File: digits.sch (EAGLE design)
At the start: 49 parts, among them IC1 STP16CP05 / STP16CPC26, IC2 STP16CP05 / STP16CPC26, IC3 ATMEGA32U4QFN, IC4 ATMEGA32U4TQFP-44, J1 POWER_JACKPTH_LOCK, J2 ACCESSORY, X1 CRYSTALHC49

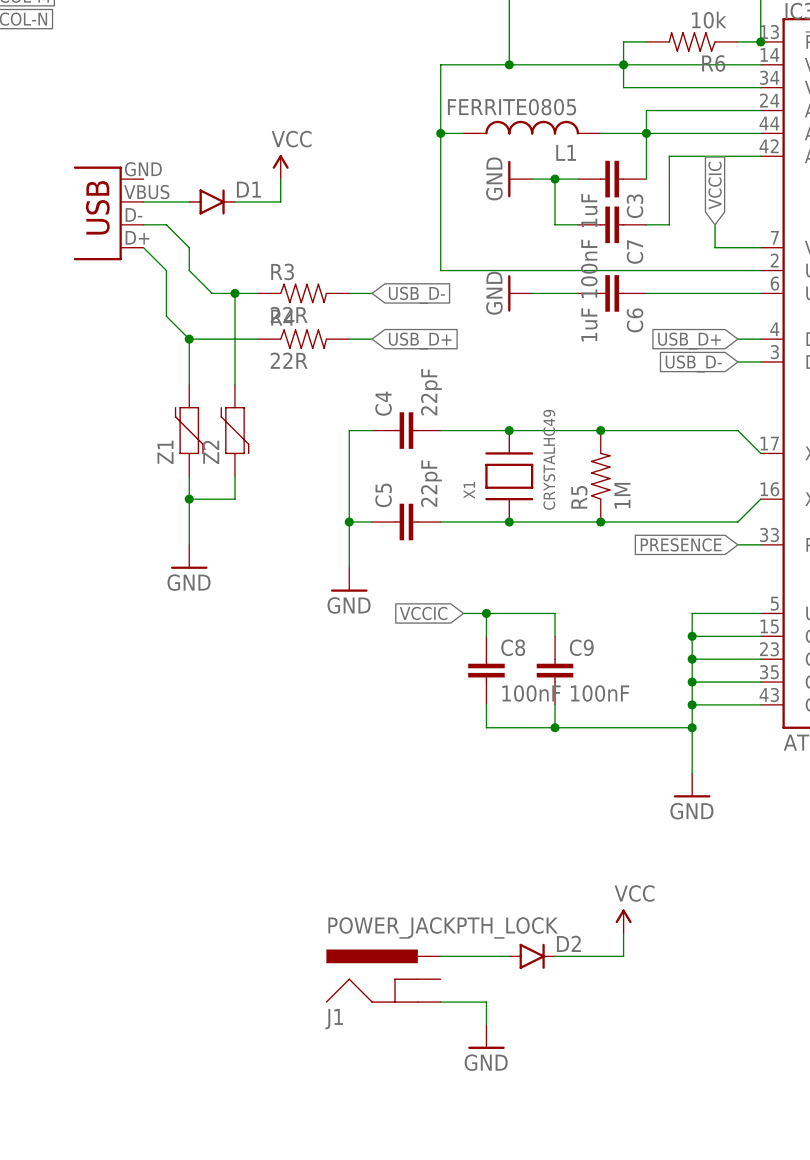
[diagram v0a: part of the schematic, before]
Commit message: finished BOM
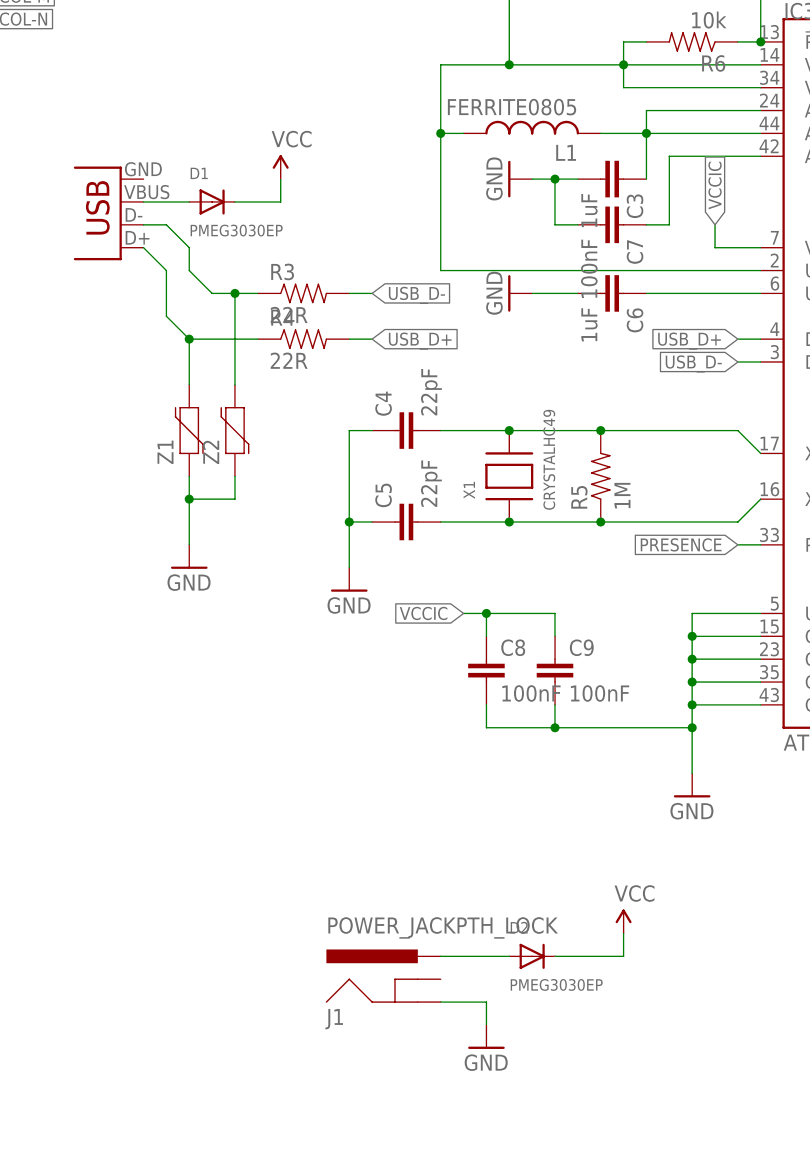
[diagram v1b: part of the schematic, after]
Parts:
- C1, C2, C7, C8, C9: PARTNO (none) -> C0805C104K5RACTU
- C3, C6: PARTNO (none) -> CL21B105KBFNNNE
- C4, C5: PARTNO (none) -> C0805C220J5GACTU
- D1, D2: value (none) -> PMEG3030EP; device SparkFun-DiscreteSemi:DIODESOD -> digits:DIODESOD-128; PARTNO (none) -> PMEG3030EP-115
- IC1, IC2: PARTNO (none) -> STP16CPC26MTR
- IC3: PARTNO (none) -> ATMEGA32U4-MUR
- IC4: PARTNO (none) -> ATMEGA32U4-AU
- J1: PARTNO (none) -> PJ-202A
- J2: PARTNO (none) -> SFH11-PBPC-D13-ST-BK
- JP1: PARTNO (none) -> M20-9980346
- JP2: PARTNO (none) -> 690-005-299-043
- JP3, JP6: PARTNO (none) -> 302-S101
- L1: PARTNO (none) -> CIM21J601NE
- LED1: PARTNO (none) -> LG R971-KN-1
- R1: PARTNO (none) -> RC0805FR-07390RL
- R2, R8: PARTNO (none) -> MCR10ERTF9100
- R3, R4: PARTNO (none) -> RC0805FR-0722RL
- R5: PARTNO (none) -> RC0805FR-071ML
- R6: PARTNO (none) -> RC0805JR-0710KL
- SJ1, SJ2, SJ3, SJ4: BOM (none) -> EXCLUDE
- T1, T2, T3, T4, T5: PARTNO (none) -> FDN352AP
- X1: PARTNO (none) -> 9C-16.000MAAJ-T
- Z1, Z2: PARTNO (none) -> CG0603MLC-05E
